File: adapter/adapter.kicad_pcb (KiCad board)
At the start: 2 copper layers, 28 x 28 mm, 9 parts, among them U1 TPS61041DBV

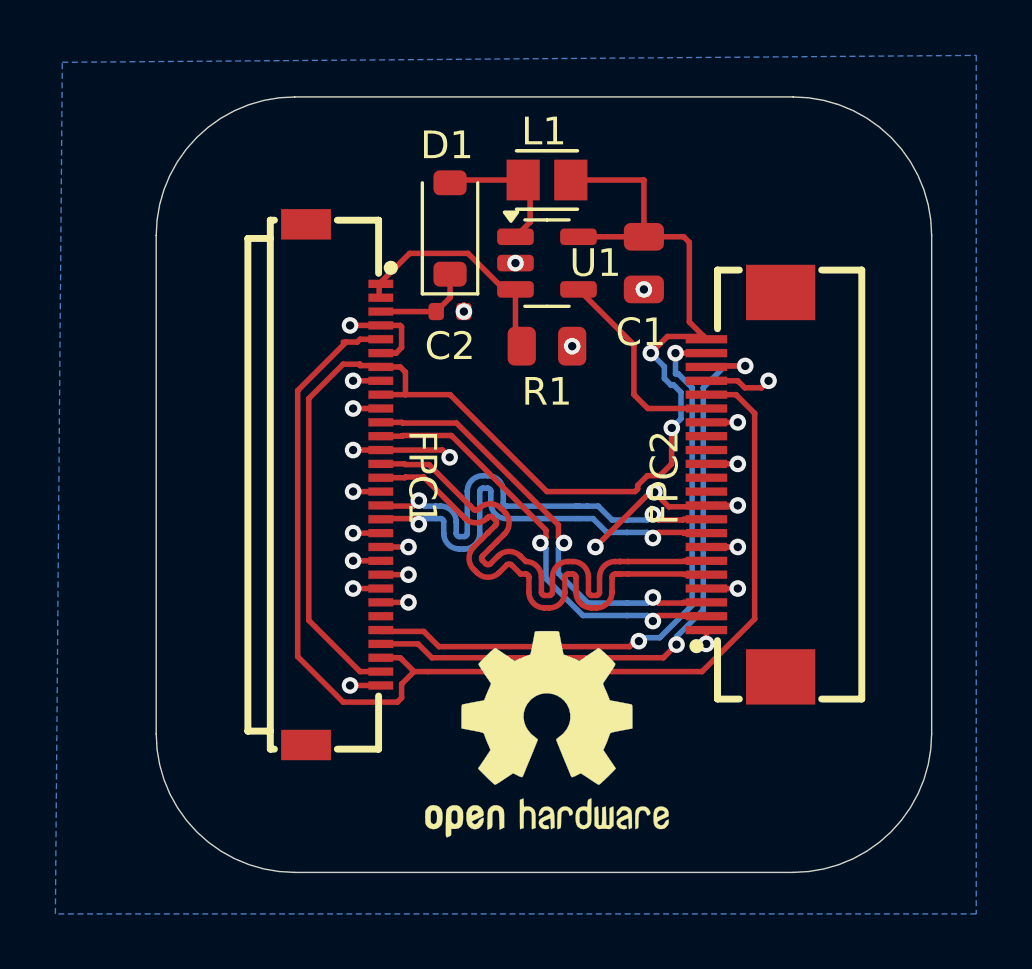
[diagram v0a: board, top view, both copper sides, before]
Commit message: WIP
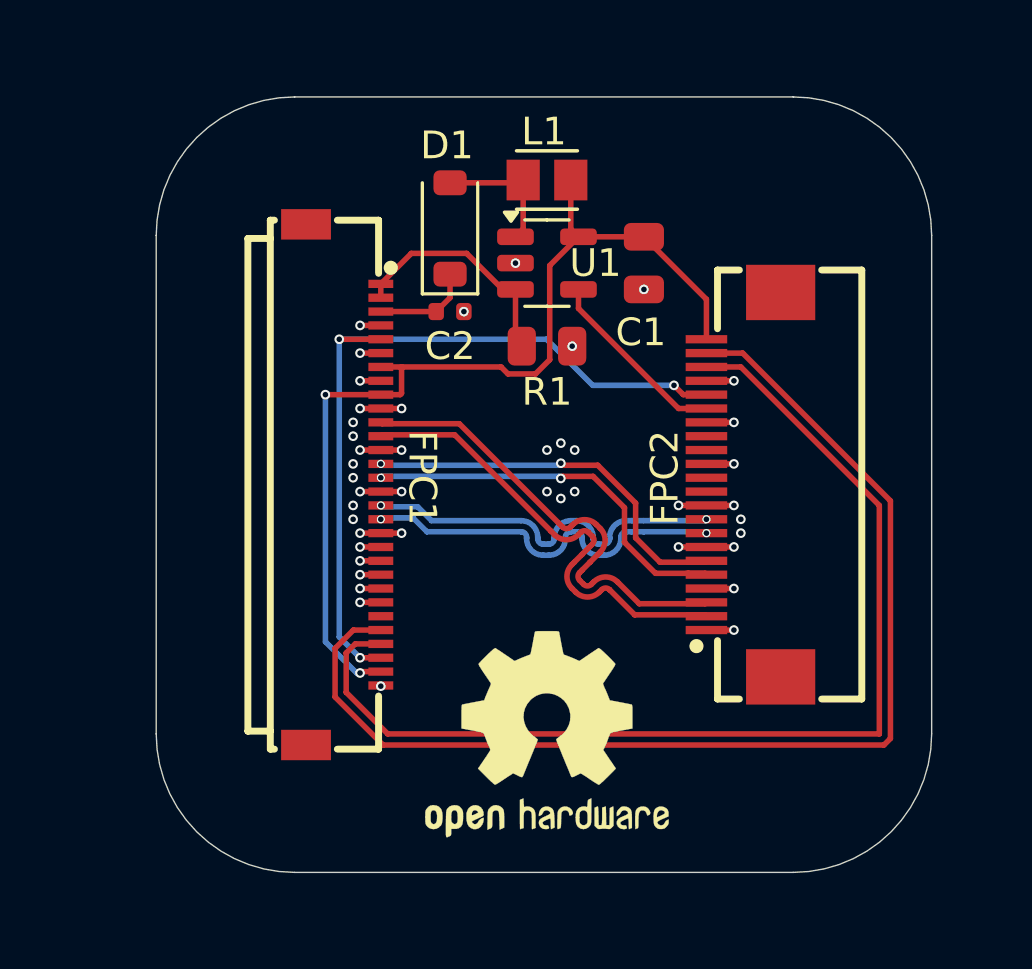
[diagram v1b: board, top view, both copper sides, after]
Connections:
- net Net-(U1-FB) renamed /CATHODE
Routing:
- net /SDA: track 23.0 -> 42.0 mm, vias 2 -> 0
- net /SCL: track 24.1 -> 39.2 mm, vias 2 -> 0
- net /RESET: track 43.1 -> 28.1 mm, vias 0 -> 3
- net /VCC: track 48.1 -> 35.6 mm
- net GND: track 32.4 -> 21.0 mm, vias 26 -> 44
- net /DSI_1_P: track 19.8 -> 14.8 mm, vias 0 -> 2
- net /DSI_1_N: track 19.8 -> 14.8 mm, vias 0 -> 2
- net /DSI_CLK_P: track 16.3 -> 14.0 mm
- net /DSI_CLK_N: track 15.9 -> 14.1 mm
- net /DSI_0_P: track 15.9 -> 17.1 mm, vias 2 -> 0
- net /DSI_0_N: track 15.9 -> 17.1 mm, vias 2 -> 0
- net /PWM: track 7.46 -> 6.80 mm
- added copper zone on In1.Cu, net GND
- added copper zone on In2.Cu, net GND
- removed copper zone on B.Cu, net GND
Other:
- copper layers 2 -> 4
